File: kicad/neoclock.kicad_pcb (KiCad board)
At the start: 2 copper layers, 45.2 x 45.2 mm, 26 parts, among them CON1 2.1mm 5V, IC1 ATMEGA328P-A, K1 NEOPIXEL, P1 ICSP, P2 FTDI, SW1 HOUR, SW2 MINUTE, U1 DS1307, X1 16Mhz, X2 32.768kHz

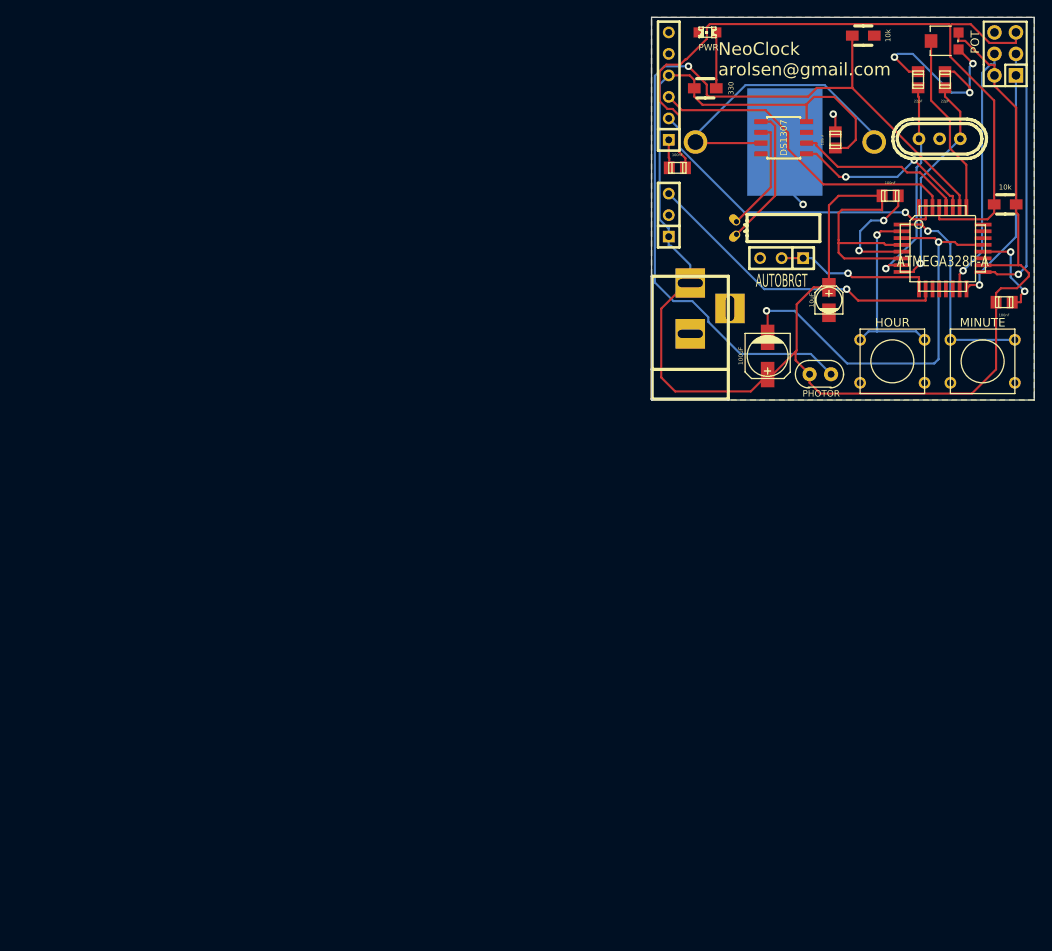
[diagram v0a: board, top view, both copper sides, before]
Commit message: updating clock board
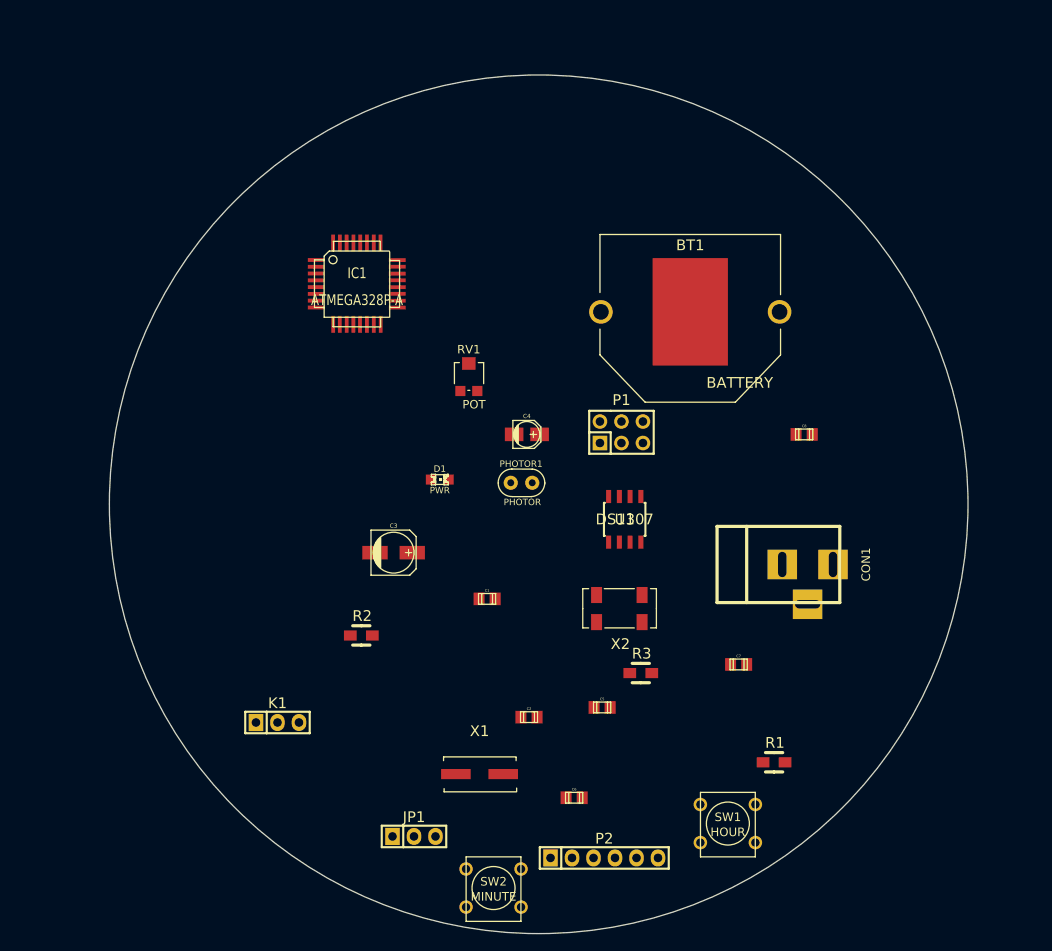
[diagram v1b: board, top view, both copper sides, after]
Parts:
- BT1: footprint WNL_CR2302_TH_KEYSTONE_3003 -> WANDL:WNL_CR2302_TH_KEYSTONE_3003; moved to F.Cu
- JP1, K1: footprint Connect:SIL-3 -> Pin_Headers:Pin_Header_Straight_1x03
- P2: footprint Connect:SIL-6 -> Pin_Headers:Pin_Header_Straight_1x06
- PHOTOR1: footprint synic:PHOTORESISTOR -> PHOTORESISTOR
- SW1, SW2: footprint Discret:SW_PUSH_SMALL -> synic:SW_PUSH_SMALL
- X1: footprint Crystals:Crystal_HC49-U_Vertical_3Pin -> synic:Crystal_HC49-SMALL_SMD
- X2: footprint Crystals:Crystal_Round_Horizontal_3mm_BigPad -> Crystal-4pad
- moved C6 95.5 mm to (87.4, 108.0), turned to 0 degrees
- moved X1 92.7 mm to (76.2, 105.2)
- moved R2 91.5 mm to (62.2, 88.8), turned to 0 degrees
- moved P2 91.5 mm to (90.9, 115.1), turned to 0 degrees
- moved SW2 84.9 mm to (77.9, 118.6)
- moved C5 83.0 mm to (90.7, 97.3), turned to 0 degrees
- moved JP1 81.0 mm to (68.5, 112.5), turned to 0 degrees
- moved R1 80.0 mm to (111.0, 103.8)
- moved R3 79.8 mm to (95.2, 93.2)
- moved K1 75.7 mm to (52.3, 99.1), turned to 0 degrees
- moved C2 74.5 mm to (82.0, 98.4)
- moved IC1 69.3 mm to (61.7, 47.2)
- moved RV1 68.9 mm to (74.9, 58.3), turned to 0 degrees
- moved C1 68.1 mm to (77.1, 84.5), turned to 0 degrees
- moved P1 63.7 mm to (93.0, 64.8), turned to 0 degrees
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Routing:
- net VCC: track 225.4 -> 0.00 mm
- net Net-(IC1-Pad26): track 102.0 -> 0.00 mm, vias 1 -> 0
- net GND: track 99.7 -> 0.00 mm, vias 9 -> 0
- net Net-(C8-Pad2): track 93.0 -> 0.00 mm
- net FTDI3: track 38.5 -> 0.00 mm
- net FTDI2: track 37.9 -> 0.00 mm, vias 1 -> 0
- net Net-(IC1-Pad10): track 37.0 -> 0.00 mm, vias 1 -> 0
- net Net-(BT1-Pad1): track 35.5 -> 0.00 mm
- net Net-(IC1-Pad17): track 31.8 -> 0.00 mm, vias 1 -> 0
- net Net-(IC1-Pad15): track 29.7 -> 0.00 mm, vias 1 -> 0
- net Net-(IC1-Pad16): track 28.3 -> 0.00 mm, vias 1 -> 0
- net Net-(C6-Pad2): track 26.2 -> 0.00 mm, vias 1 -> 0
- net Net-(IC1-Pad1): track 25.6 -> 0.00 mm, vias 1 -> 0
- net Net-(C5-Pad2): track 25.3 -> 0.00 mm, vias 1 -> 0
- net Net-(IC1-Pad2): track 23.0 -> 0.00 mm, vias 1 -> 0
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- removed copper zone on B.Cu, net GND
- removed copper zone on F.Cu, net GND
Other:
- board size 45.2 x 45.2 mm -> 101.4 x 101.4 mm
- board text removed: "NeoClock arolsen@gmail.com"

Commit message: updates
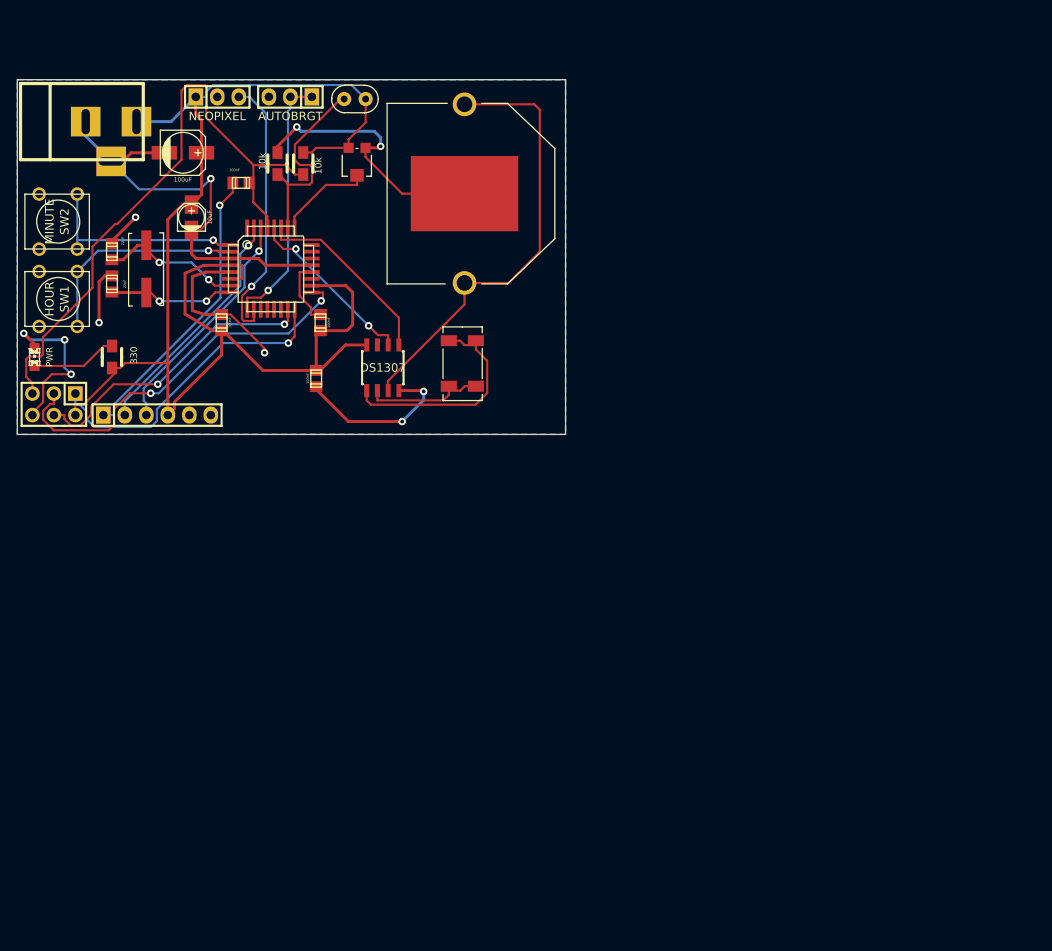
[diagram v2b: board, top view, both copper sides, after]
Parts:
- BT1: footprint WANDL:WNL_CR2302_TH_KEYSTONE_3003 -> synic:WNL_CR2302_TH_KEYSTONE_3003
- moved SW1 100.5 mm to (26.4, 49.0), turned to 270 degrees
- moved CON1 97.5 mm to (29.5, 28.1)
- moved SW2 94.1 mm to (26.4, 39.9), turned to 270 degrees
- moved R1 91.7 mm to (32.8, 55.9), turned to 90 degrees
- moved JP1 88.6 mm to (53.8, 25.1), turned to 180 degrees
- moved C6 81.7 mm to (32.8, 47.2), turned to 90 degrees
- moved C5 79.1 mm to (32.8, 43.4), turned to 90 degrees
- moved P2 74.4 mm to (38.1, 62.7)
- moved K1 74.3 mm to (45.2, 25.1)
- moved R3 73.9 mm to (52.3, 33.0), turned to 90 degrees
- moved C7 73.2 mm to (45.7, 51.8), turned to 90 degrees
- moved C8 72.9 mm to (48.0, 35.3), turned to 180 degrees
- moved X1 71.5 mm to (36.8, 45.5), turned to 270 degrees
- moved P1 67.1 mm to (25.9, 61.5), turned to 180 degrees
- moved R2 56.2 mm to (55.4, 33.0), turned to 270 degrees
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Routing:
- net VCC: track 0.00 -> 167.8 mm
- net GND: track 0.00 -> 153.1 mm, vias 0 -> 11
- net Net-(C8-Pad2): track 0.00 -> 74.5 mm
- net Net-(BT1-Pad1): track 0.00 -> 52.8 mm
- net Net-(IC1-Pad17): track 0.00 -> 47.1 mm, vias 0 -> 2
- net Net-(IC1-Pad16): track 0.00 -> 37.3 mm, vias 0 -> 1
- net Net-(IC1-Pad15): track 0.00 -> 35.5 mm, vias 0 -> 2
- net Net-(C8-Pad1): track 0.00 -> 34.6 mm, vias 0 -> 1
- net Net-(IC1-Pad10): track 0.00 -> 32.4 mm, vias 0 -> 1
- net Net-(IC1-Pad9): track 0.00 -> 30.7 mm, vias 0 -> 1
- net FTDI2: track 0.00 -> 28.4 mm, vias 0 -> 1
- net FTDI3: track 0.00 -> 27.9 mm, vias 0 -> 1
- net Net-(U1-Pad1): track 0.00 -> 26.3 mm
- net Net-(IC1-Pad2): track 0.00 -> 25.7 mm, vias 0 -> 1
- net Net-(IC1-Pad1): track 0.00 -> 24.8 mm, vias 0 -> 1
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- added copper zone on B.Cu, net GND
- added copper zone on F.Cu, net GND
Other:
- board size 101.4 x 101.4 mm -> 64.8 x 41.9 mm
- rule trace_min: 0.254 -> 0.2
- board text added: "NeoClock v0 by Adam Olsen arolsen@gmail.com"
